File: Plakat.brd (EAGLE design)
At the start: 82.4 x 68.1 mm, 25 parts, among them X1 USB-MICROB

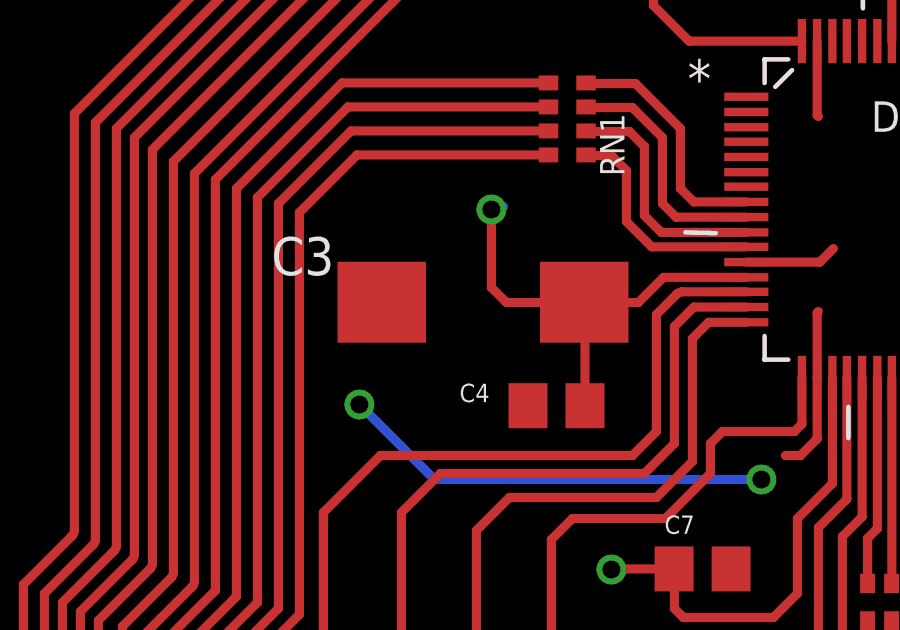
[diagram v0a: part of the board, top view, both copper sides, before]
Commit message: Nothing
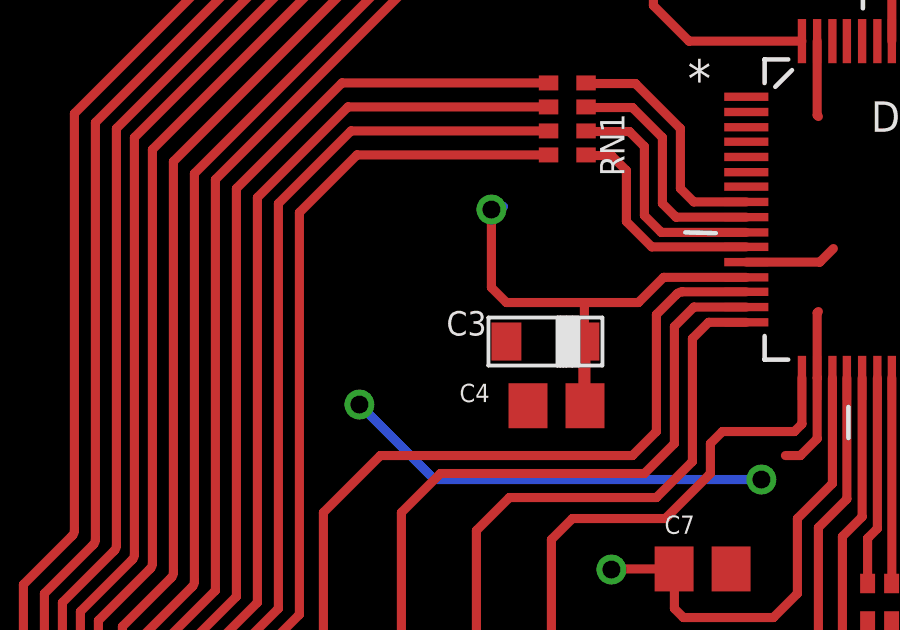
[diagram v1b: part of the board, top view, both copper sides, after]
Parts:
- C3: device resistor:D/7343-31W -> rcl:TYPE_A_TECAP
- moved C3 1.97 mm to (65.7, 51.5)
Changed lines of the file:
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@@
 <attribute name="VALUE" x="108.97" y="56.35" size="0.8128" layer="27" rot="R270"/>
-</element>
-<element name="C3" library="resistor" package="D/7343-31W" value="1uF" x="65.22" y="53.41" smashed="yes">
-<attribute name="NAME" x="58.17" y="54.31" size="1.27" layer="25"/>
-<attribute name="VALUE" x="57.07" y="52.135" size="1.27" layer="27"/>
 </element>
 <element name="C4" library="rcl" package="C0805" value="100nF" x="67.67" y="49.96" smashed="yes" rot="R180">
@@
 <element name="X4" library="pinhead" package="2X20" value="" x="84.57" y="21.57" rot="R180"/>
 <element name="L1" library="BOURNS" package="101KL" value="100uH" x="116.9" y="33.1" rot="R90"/>
+<element name="C3" library="rcl" package="TYPE_A_TECAP" value="1uF" x="65.7" y="51.5" smashed="yes">
+<attribute name="NAME" x="64" y="52.3" size="0.8128" layer="25"/>
+<attribute name="VALUE" x="63.4" y="51.2" size="0.8128" layer="27"/>
+</element>
 </elements>
 <signals>
@@
 <contactref element="5V" pad="C"/>
 <contactref element="C4" pad="2"/>
-<contactref element="C3" pad="-"/>
 <contactref element="C5" pad="2"/>
 <contactref element="C8" pad="2"/>
@@
 <wire x1="75.8" y1="48.3" x2="75.3" y2="48.3" width="0.3048" layer="1"/>
 <wire x1="76.3588" y1="48.8588" x2="75.8" y2="48.3" width="0.3048" layer="1"/>
+<contactref element="C3" pad="-"/>
 </signal>
 <signal name="N$2">
@@
 <contactref element="DA1" pad="FB"/>
 <contactref element="C4" pad="1"/>
-<contactref element="C3" pad="+"/>
 <contactref element="C5" pad="1"/>
 <contactref element="C6" pad="1"/>
@@
 <wire x1="75.8508" y1="62.1134" x2="72.0866" y2="62.1134" width="0.3048" layer="1"/>
 <wire x1="72.0866" y1="62.1134" x2="70.9" y2="63.3" width="0.3048" layer="1"/>
-<wire x1="68.62" y1="49.96" x2="68.62" y2="53.385" width="0.3048" layer="1"/>
 <wire x1="68.62" y1="53.385" x2="68.605" y2="53.4" width="0.3048" layer="1"/>
 <wire x1="113.115" y1="54.185" x2="112.085" y2="54.185" width="0.3048" layer="1"/>
@@
 <wire x1="65.8" y1="56.5" x2="65.9" y2="56.6" width="0.3048" layer="16"/>
 <wire x1="70.4" y1="53.4" x2="68.605" y2="53.4" width="0.3048" layer="1"/>
-<wire x1="68.605" y1="53.4" x2="68.595" y2="53.41" width="0.3048" layer="1"/>
 <wire x1="71.59" y1="44.52" x2="69.52" y2="44.52" width="0.3048" layer="1"/>
 <wire x1="69.52" y1="44.52" x2="69.5" y2="44.5" width="0.3048" layer="1"/>
@@
 <wire x1="85.5" y1="50.7" x2="85.5" y2="49.43" width="0.3048" layer="1"/>
 <wire x1="85.5" y1="49.43" x2="85.49" y2="49.42" width="0.3048" layer="1"/>
+<contactref element="C3" pad="+"/>
+<wire x1="68.62" y1="49.96" x2="68.6" y2="49.96" width="0.4064" layer="1"/>
+<wire x1="68.6" y1="49.96" x2="68.6" y2="52.1" width="0.4064" layer="1"/>
+<wire x1="68.6" y1="52.1" x2="68.6" y2="53.395" width="0.3048" layer="1"/>
+<wire x1="68.6" y1="53.395" x2="68.605" y2="53.4" width="0.3048" layer="1"/>
 </signal>
 <signal name="N$3">
